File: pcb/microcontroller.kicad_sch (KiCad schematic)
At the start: 14 parts, among them IC5 ESP32-C3-MINI-1-N4

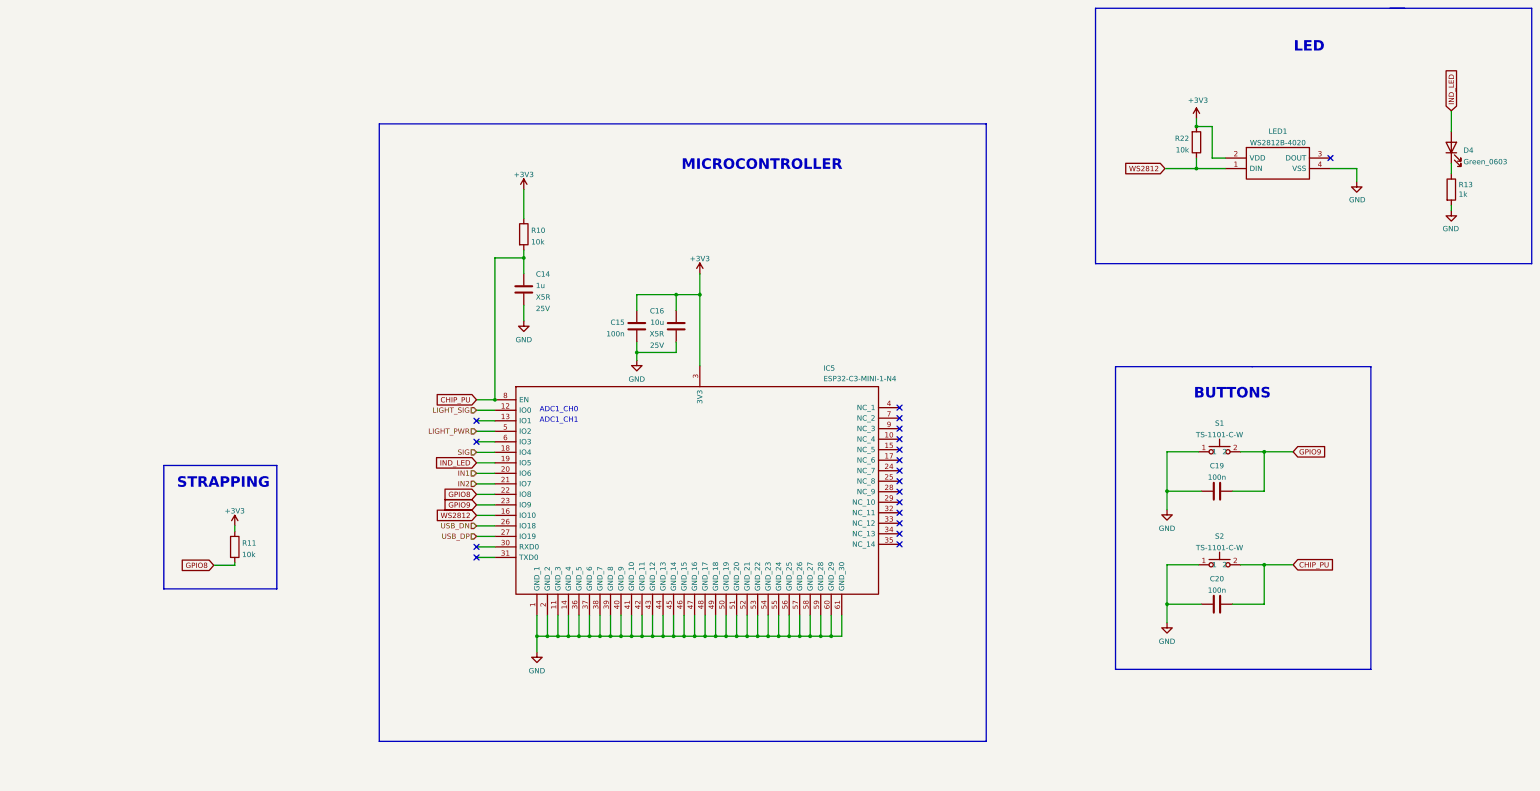
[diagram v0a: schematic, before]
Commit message: Completed initial schematic
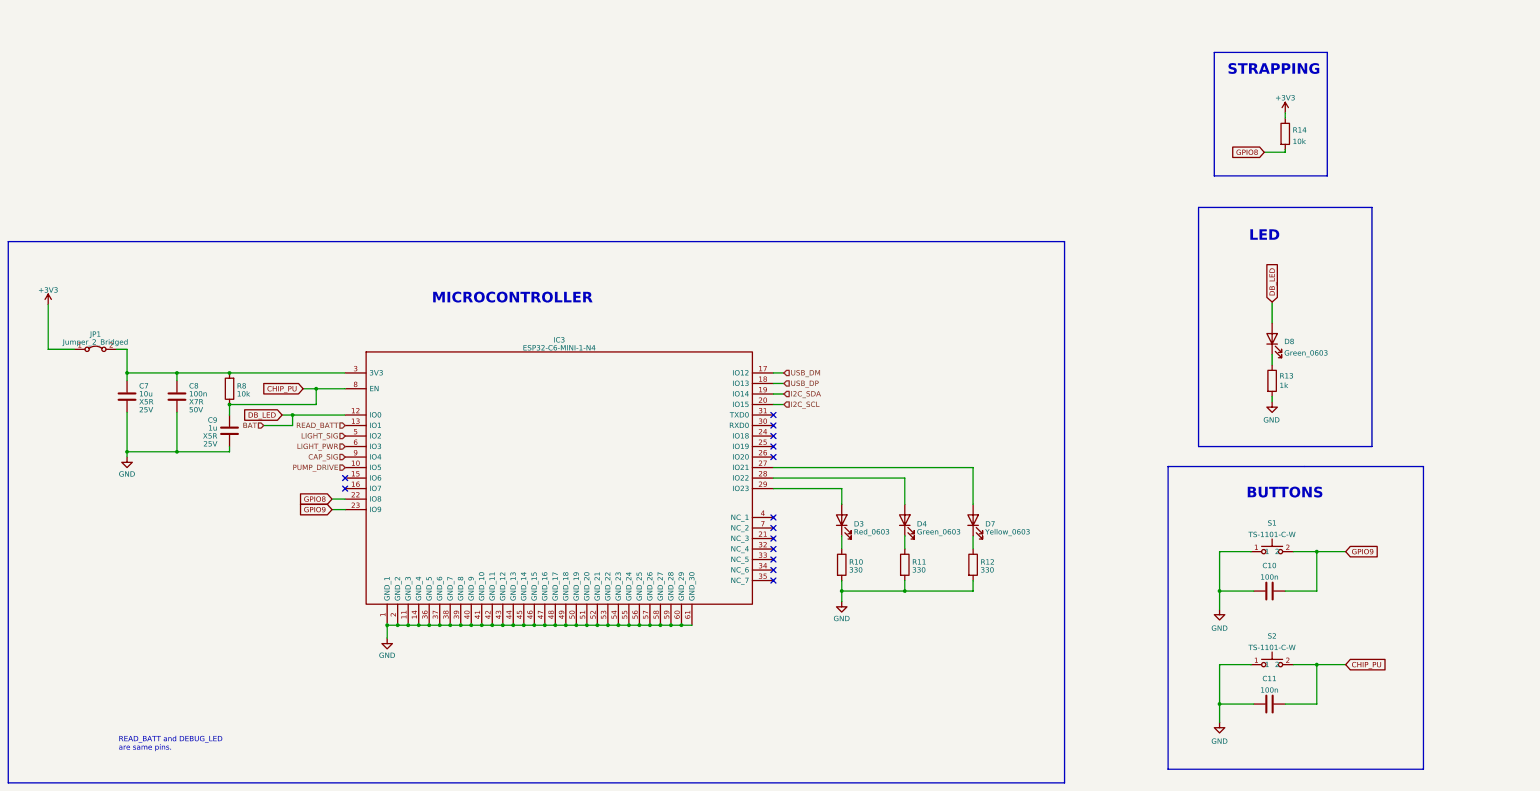
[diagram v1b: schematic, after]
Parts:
- removed C14: 1u, Capacitor_SMD:C_0402_1005Metric, symbol Capacitor_JLC:1u
- removed C15, C19, C20: 100n, Capacitor_SMD:C_0402_1005Metric, symbol Capacitor_JLC:100n
- removed C16: 10u, Capacitor_SMD:C_0805_2012Metric, symbol Capacitor_JLC:10u
- removed IC5: ESP32-C3-MINI-1-N4, ESP32C3MINI1N4, symbol MCU_JLC:ESP32-C3-MINI-1-N4
- removed LED1: WS2812B-4020, WS2812B4020, symbol Diode_JLC:WS2812B-4020
- removed R10, R11, R22: 10k, Resistor_SMD:R_0402_1005Metric, symbol Resistor_JLC:10k
- added C10, C11, C8: 100n, Capacitor_SMD:C_0402_1005Metric, symbol Capacitor_JLC:100n
- added C7: 10u, Capacitor_SMD:C_0805_2012Metric, symbol Capacitor_JLC:10u
- added C9: 1u, Capacitor_SMD:C_0402_1005Metric, symbol Capacitor_JLC:1u
- added D3: Red_0603, LED_SMD:LED_0603_1608Metric, symbol Diode_JLC:Red_0603
- added D7: Yellow_0603, LED_SMD:LED_0603_1608Metric, symbol Diode_JLC:Yellow_0603
- added D8: Green_0603, LED_SMD:LED_0603_1608Metric, symbol Diode_JLC:Green_0603
- added IC3: ESP32-C6-MINI-1-N4, ESP32C6MINI1N4, symbol MCU_JLC:ESP32-C6-MINI-1-N4
- added JP1: Jumper_2_Bridged, Jumper:SolderJumper-2_P1.3mm_Bridged_RoundedPad1.0x1.5mm, symbol Jumper:Jumper_2_Bridged
- added R10, R11, R12: 330, Resistor_SMD:R_0402_1005Metric, symbol Resistor_JLC:330
- added R14, R8: 10k, Resistor_SMD:R_0402_1005Metric, symbol Resistor_JLC:10k
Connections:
- net +3V3: now also JP1.1 (A), R14.1
- net CHIP_PU: now also C11.2, C9.2, IC3.8 (EN), R8.1
- net GND: now also C10.1, C11.1, C7.2, C8.2, C9.1, IC3.1 (GND_1), IC3.11 (GND_3), IC3.14 (GND_4), IC3.2 (GND_2), IC3.36 (GND_5), IC3.37 (GND_6), IC3.38 (GND_7), IC3.39 (GND_8), IC3.40 (GND_9), IC3.41 (GND_10), IC3.42 (GND_11), IC3.43 (GND_12), IC3.44 (GND_13), IC3.45 (GND_14), IC3.46 (GND_15), IC3.47 (GND_16), IC3.48 (GND_17), IC3.49 (GND_18), IC3.50 (GND_19), IC3.51 (GND_20), IC3.52 (GND_21), IC3.53 (GND_22), IC3.54 (GND_23), IC3.55 (GND_24), IC3.56 (GND_25), IC3.57 (GND_26), IC3.58 (GND_27), IC3.59 (GND_28), IC3.60 (GND_29), IC3.61 (GND_30), R10.2, R11.2, R12.2
- net GPIO8: now also IC3.22 (IO8), R14.2
- net GPIO9: now also C10.2, IC3.23 (IO9)
- net LIGHT_PWR: now also IC3.6 (IO3)
- net LIGHT_SIG: now also IC3.5 (IO2)
- net USB_DP: now also IC3.18 (IO13)
- net at D4.1 (K): now also R11.1; no longer R13.1
- net IND_LED: no longer names the net of D4.2 (A)
- net IND_LED: now also IC3.28 (IO22)
- new net: C7.1, C8.1, IC3.3 (3V3), JP1.2 (B), R8.2
- new net: D7.1 (K), R12.1
- new net: D7.2 (A), IC3.27 (IO21)
- new net: D3.1 (K), R10.1
- new net: D3.2 (A), IC3.29 (IO23)
- new net: D8.1 (K), R13.1
- new net CAP_SIG: IC3.9 (IO4)
- new net DB_LED: D8.2 (A), IC3.12 (IO0)
- new net I2C_SCL: IC3.20 (IO15)
- new net I2C_SDA: IC3.19 (IO14)
- new net PUMP_DRIVE: IC3.10 (IO5)
- new net READ_BATT: IC3.13 (IO1)
- new net USB_DM: IC3.17 (IO12)
- no-connect marks 19 -> 14
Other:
- note added: "READ_BATT and DEBUG_LED are same pins."
- note removed: "ADC1_CH0"
- note removed: "ADC1_CH1"
